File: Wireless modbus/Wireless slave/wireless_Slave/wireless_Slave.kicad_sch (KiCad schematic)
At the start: 0 parts

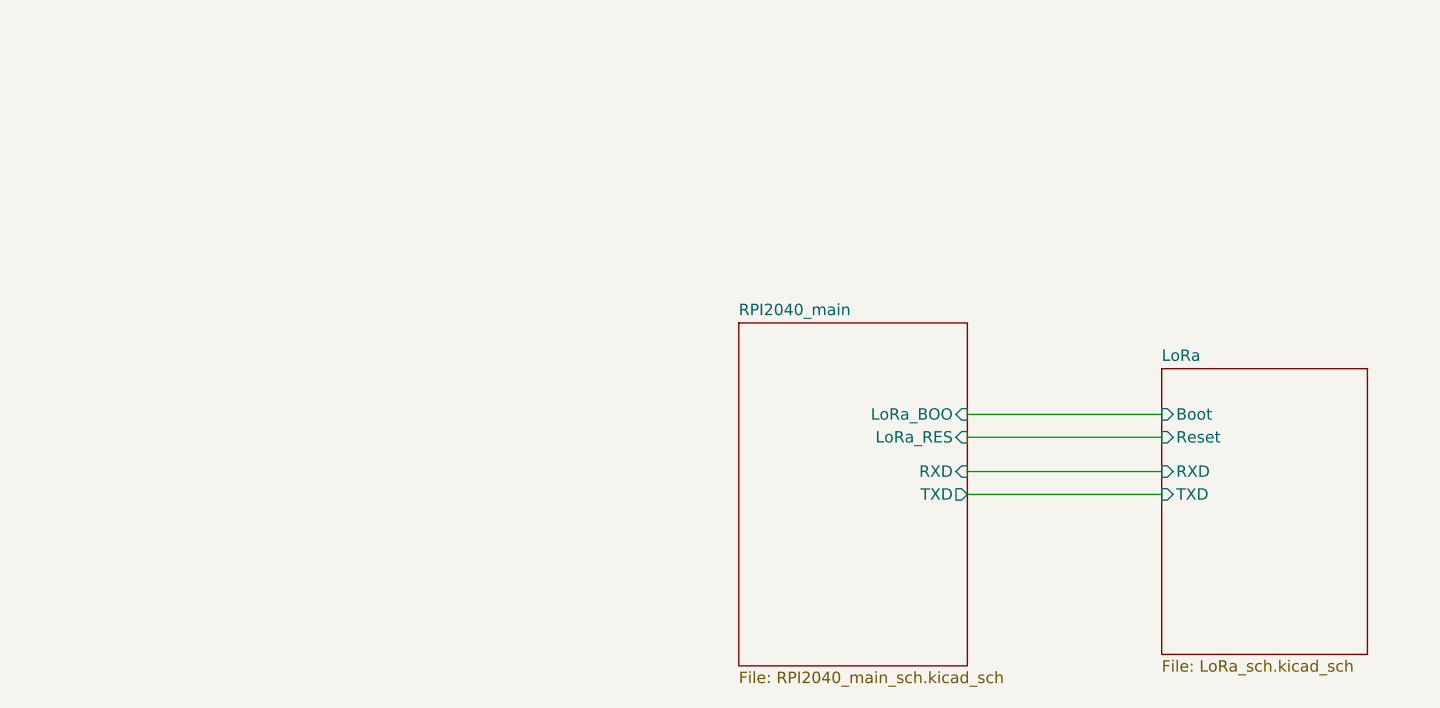
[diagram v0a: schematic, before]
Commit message: Ændring
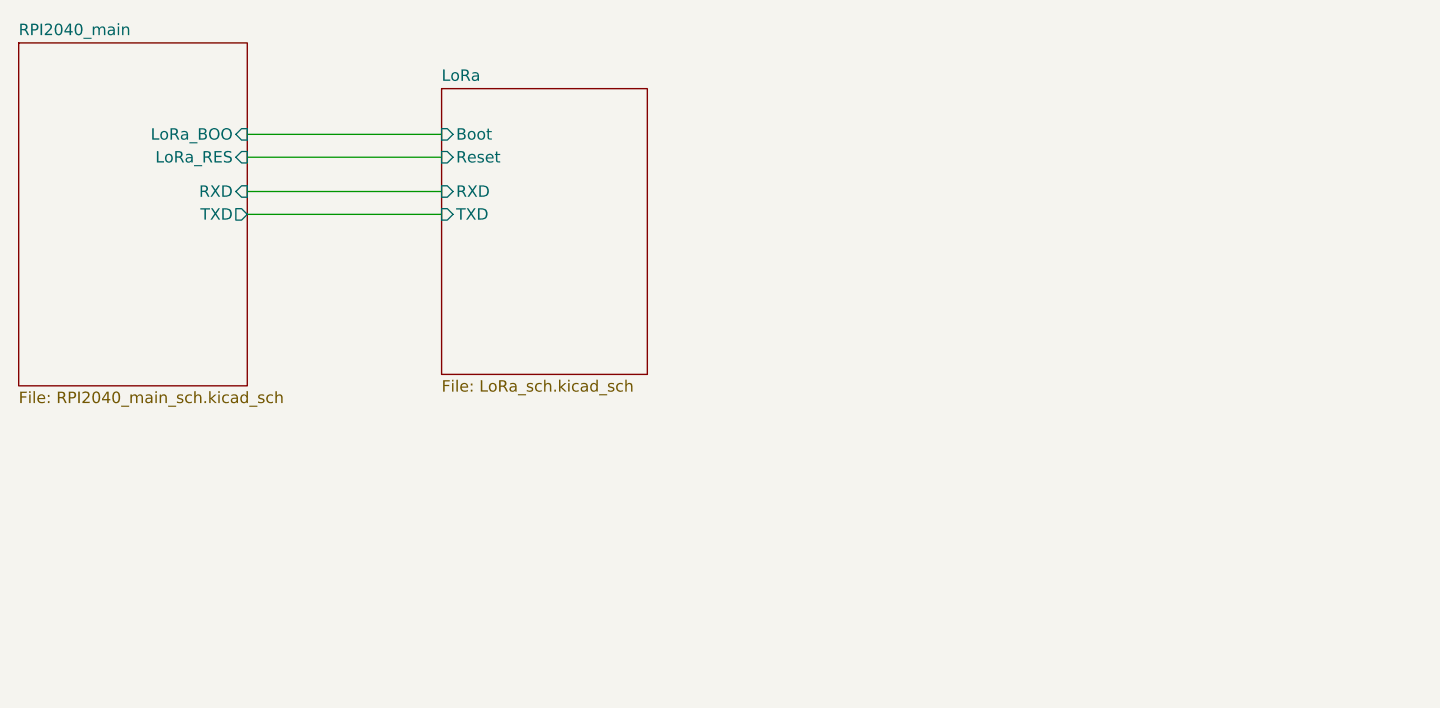
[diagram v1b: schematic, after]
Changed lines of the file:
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@@
 (kicad_sch (version 20230121) (generator eeschema)
   (paper "A4")
-  (wire (pts (xy 177.8 73.66) (xy 199.39 73.66))
+  (wire (pts (xy 97.79 42.545) (xy 119.38 42.545))
     (stroke (width 0) (type default))
   )
-  (wire (pts (xy 177.8 80.01) (xy 199.39 80.01))
+  (wire (pts (xy 97.79 48.895) (xy 119.38 48.895))
     (stroke (width 0) (type default))
   )
-  (wire (pts (xy 177.8 76.2) (xy 199.39 76.2))
+  (wire (pts (xy 97.79 45.085) (xy 119.38 45.085))
     (stroke (width 0) (type default))
   )
-  (wire (pts (xy 177.8 82.55) (xy 199.39 82.55))
+  (wire (pts (xy 97.79 51.435) (xy 119.38 51.435))
     (stroke (width 0) (type default))
   )
-  (sheet (at 152.4 63.5) (size 25.4 38.1) (fields_autoplaced)
+  (sheet (at 72.39 32.385) (size 25.4 38.1) (fields_autoplaced)
     (stroke (width 0.1524) (type solid))
     (fill (color 0 0 0 0.0000))
-    (property "Sheetname" "RPI2040_main" (at 152.4 62.7884 0)
+    (property "Sheetname" "RPI2040_main" (at 72.39 31.6734 0)
       (effects (font (size 1.27 1.27)) (justify left bottom))
     )
-    (property "Sheetfile" "RPI2040_main_sch.kicad_sch" (at 152.4 102.1846 0)
+    (property "Sheetfile" "RPI2040_main_sch.kicad_sch" (at 72.39 71.0696 0)
       (effects (font (size 1.27 1.27)) (justify left top))
     )
-    (pin "RXD" input (at 177.8 80.01 0)
+    (pin "RXD" input (at 97.79 48.895 0)
       (effects (font (size 1.27 1.27)) (justify right))
     )
-    (pin "TXD" output (at 177.8 82.55 0)
+    (pin "TXD" output (at 97.79 51.435 0)
       (effects (font (size 1.27 1.27)) (justify right))
     )
-    (pin "LoRa_BOO" input (at 177.8 73.66 0)
+    (pin "LoRa_BOO" input (at 97.79 42.545 0)
       (effects (font (size 1.27 1.27)) (justify right))
     )
-    (pin "LoRa_RES" input (at 177.8 76.2 0)
+    (pin "LoRa_RES" input (at 97.79 45.085 0)
       (effects (font (size 1.27 1.27)) (justify right))
     )
@@
     )
   )
-  (sheet (at 199.39 68.58) (size 22.86 31.75) (fields_autoplaced)
+  (sheet (at 119.38 37.465) (size 22.86 31.75) (fields_autoplaced)
     (stroke (width 0.1524) (type solid))
     (fill (color 0 0 0 0.0000))
-    (property "Sheetname" "LoRa" (at 199.39 67.8684 0)
+    (property "Sheetname" "LoRa" (at 119.38 36.7534 0)
       (effects (font (size 1.27 1.27)) (justify left bottom))
     )
-    (property "Sheetfile" "LoRa_sch.kicad_sch" (at 199.39 100.9146 0)
+    (property "Sheetfile" "LoRa_sch.kicad_sch" (at 119.38 69.7996 0)
       (effects (font (size 1.27 1.27)) (justify left top))
     )
-    (pin "Boot" input (at 199.39 73.66 180)
+    (pin "Boot" input (at 119.38 42.545 180)
       (effects (font (size 1.27 1.27)) (justify left))
     )
-    (pin "Reset" input (at 199.39 76.2 180)
+    (pin "Reset" input (at 119.38 45.085 180)
       (effects (font (size 1.27 1.27)) (justify left))
     )
-    (pin "RXD" input (at 199.39 80.01 180)
+    (pin "RXD" input (at 119.38 48.895 180)
       (effects (font (size 1.27 1.27)) (justify left))
     )
-    (pin "TXD" input (at 199.39 82.55 180)
+    (pin "TXD" input (at 119.38 51.435 180)
       (effects (font (size 1.27 1.27)) (justify left))
     )
